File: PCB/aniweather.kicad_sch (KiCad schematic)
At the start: 4 parts, among them SW1 SW_SPDT

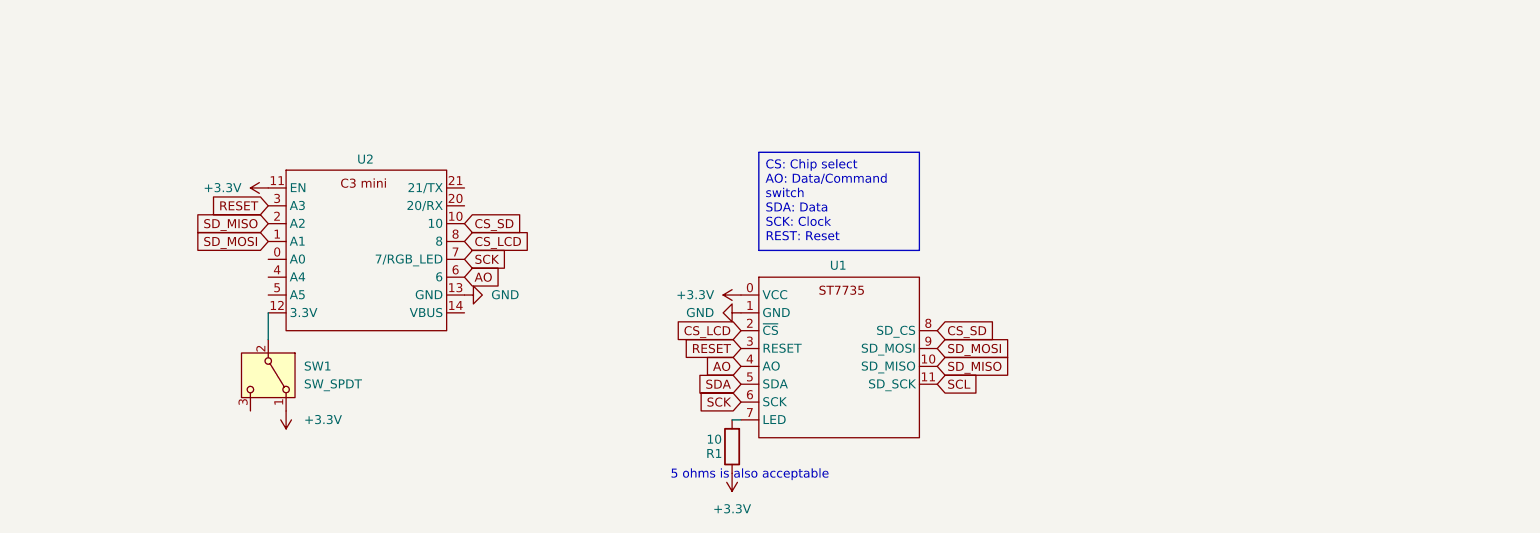
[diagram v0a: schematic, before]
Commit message: Further improvements
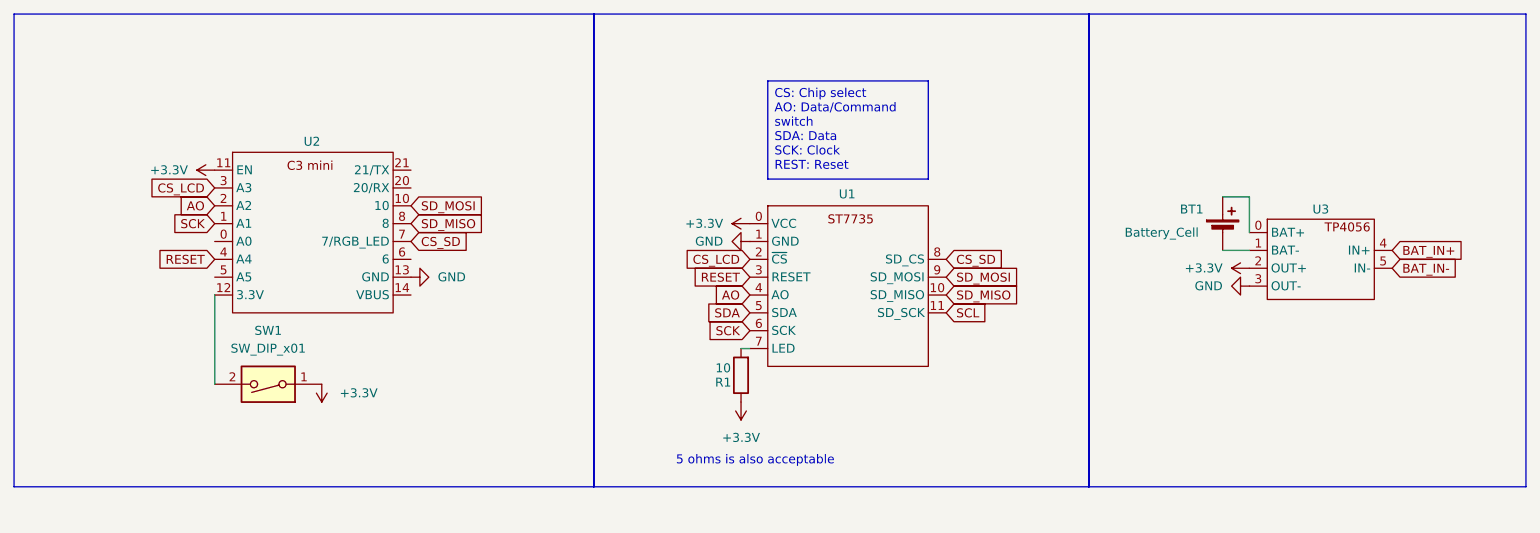
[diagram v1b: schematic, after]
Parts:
- removed SW1: SW_SPDT, symbol Switch:SW_SPDT
- added BT1: Battery_Cell, TestPoint:TestPoint_2Pads_Pitch5.08mm_Drill1.3mm, symbol Device:Battery_Cell
- added SW1: SW_DIP_x01, Button_Switch_THT:SW_DIP_SPSTx01_Slide_9.78x4.72mm_W7.62mm_P2.54mm, symbol Switch:SW_DIP_x01
- added U3: ~, asylum:TP4056, symbol asylum:TP4056
- R1: footprint (none) -> Resistor_THT:R_Axial_DIN0207_L6.3mm_D2.5mm_P10.16mm_Horizontal
- U1: footprint (none) -> asylum:ST7735
- U2: footprint (none) -> asylum:C3 mini
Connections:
- net +3.3V: now also SW1.1, U3.2 (OUT+)
- net AO: now also U2.2 (A2); no longer U2.6
- net CS_LCD: now also U2.3 (A3); no longer U2.8
- net CS_SD: now also U2.7 (7/RGB_LED); no longer U2.10
- net GND: now also U3.3 (OUT-)
- net RESET: now also U2.4 (A4); no longer U2.3 (A3)
- net SCK: now also U2.1 (A1); no longer U2.7 (7/RGB_LED)
- net SD_MISO: now also U2.8; no longer U2.2 (A2)
- net SD_MOSI: now also U2.10; no longer U2.1 (A1)
- net at U2.12 (3.3V): now also SW1.2
- new net: BT1.1 (+), U3.0 (BAT+)
- new net: BT1.2 (-), U3.1 (BAT-)
- new net BAT_IN+: U3.4 (IN+)
- new net BAT_IN-: U3.5 (IN-)
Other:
- moved on the sheet: R1, U1, U2

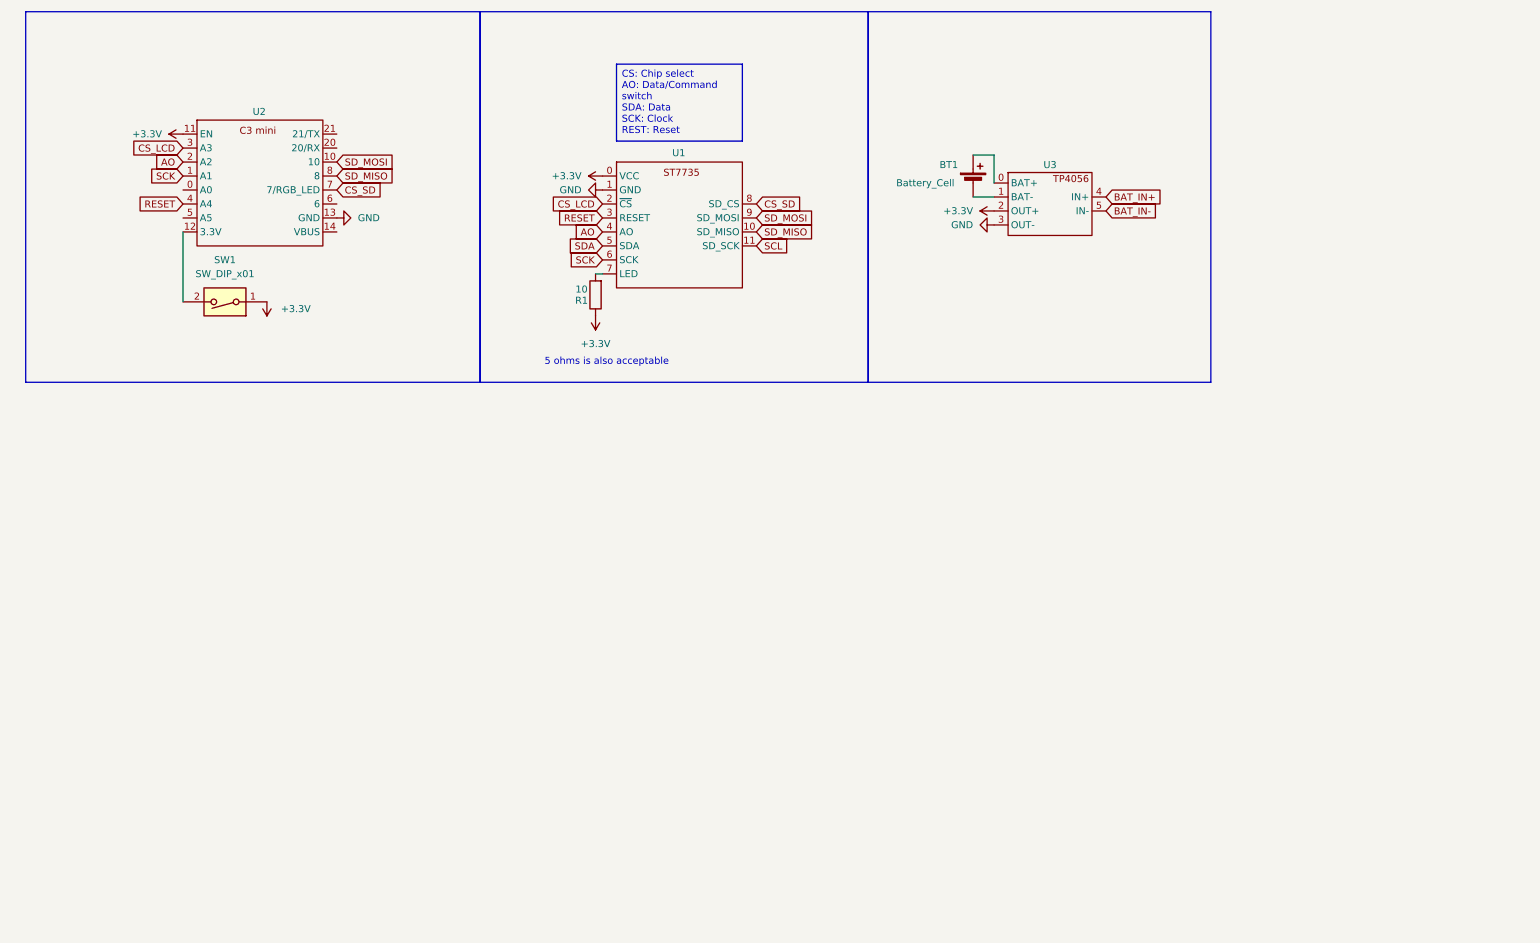
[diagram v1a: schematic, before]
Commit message: Saber plus PCB start
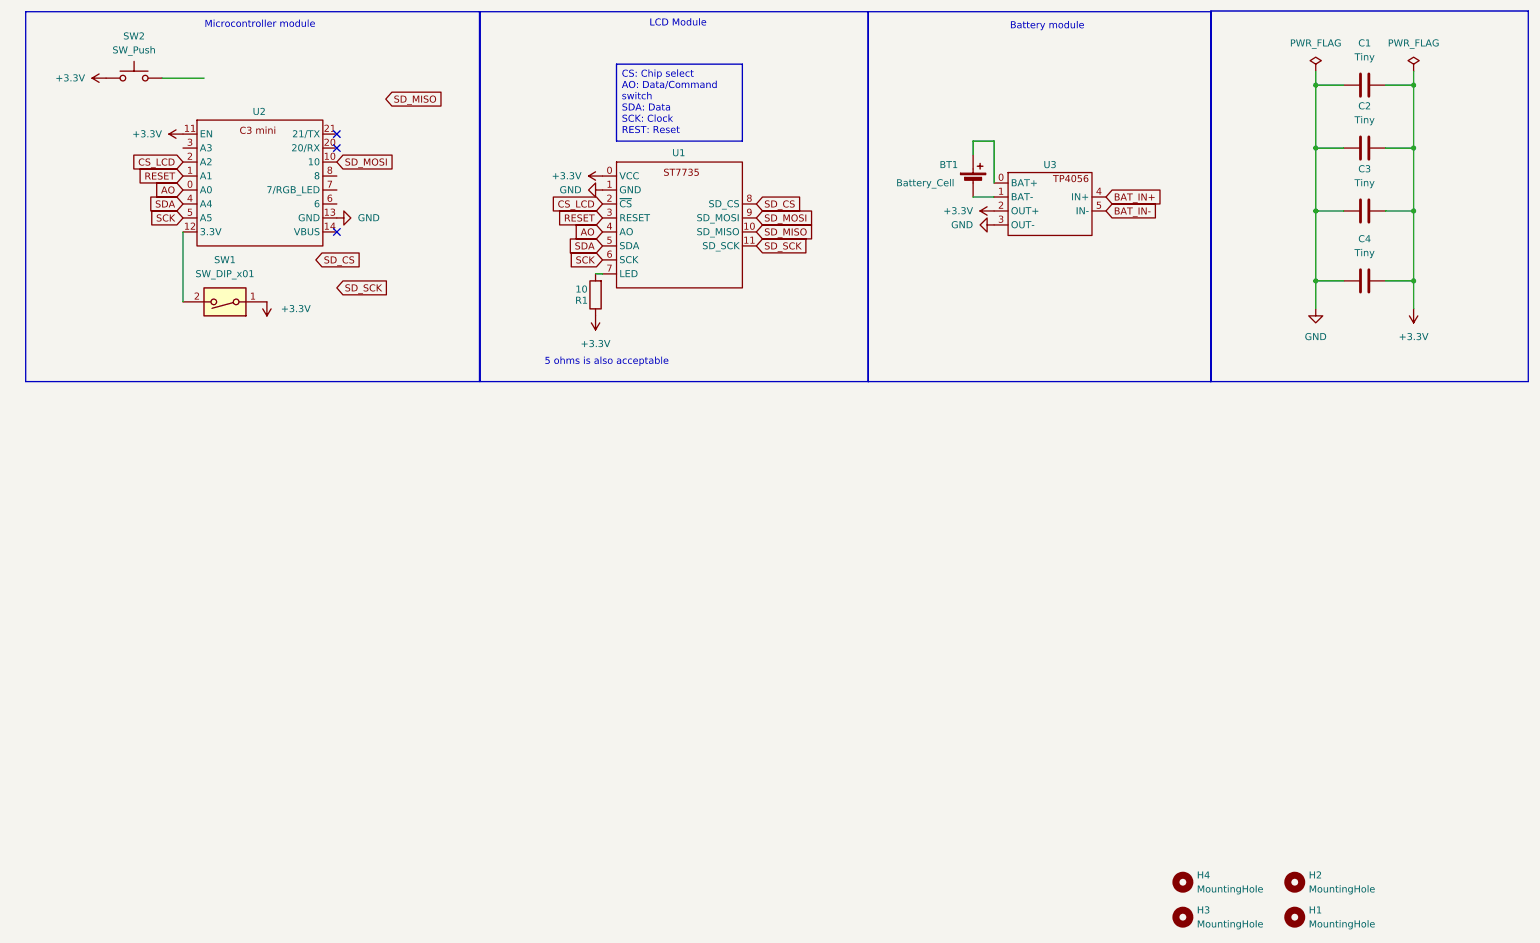
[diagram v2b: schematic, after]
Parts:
- added C1, C2, C3, C4: Tiny, Capacitor_THT:C_Disc_D5.0mm_W2.5mm_P2.50mm, symbol Device:C
- added H1, H2, H3, H4: MountingHole, MountingHole:MountingHole_3.2mm_M3, symbol Mechanical:MountingHole
- added SW2: SW_Push, Button_Switch_THT:SW_PUSH_6mm, symbol Switch:SW_Push
- U2: footprint asylum:C3 mini -> asylum:WEMOS_C1_mini
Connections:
- net +3.3V: now also C1.2, C2.2, C3.2, C4.2, SW2.1
- net AO: now also U2.0 (A0); no longer U2.2 (A2)
- net CS_LCD: now also U2.2 (A2); no longer U2.3 (A3)
- net GND: now also C1.1, C2.1, C3.1, C4.1
- net RESET: now also U2.1 (A1); no longer U2.4 (A4)
- net SCK: now also U2.5 (A5); no longer U2.1 (A1)
- net SDA: now also U2.4 (A4)
- net SD_MISO: no longer U2.8
- net CS_SD: no longer names the net of U2.7 (7/RGB_LED)
- net CS_SD: no longer U1.8 (SD_CS)
- net SCL renamed SD_SCK
- new net SD_CS: U1.8 (SD_CS)
- no-connect marks 0 -> 3
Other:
- note added: "Battery module"
- note added: "LCD Module"
- note added: "Microcontroller module"

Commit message: V1.0
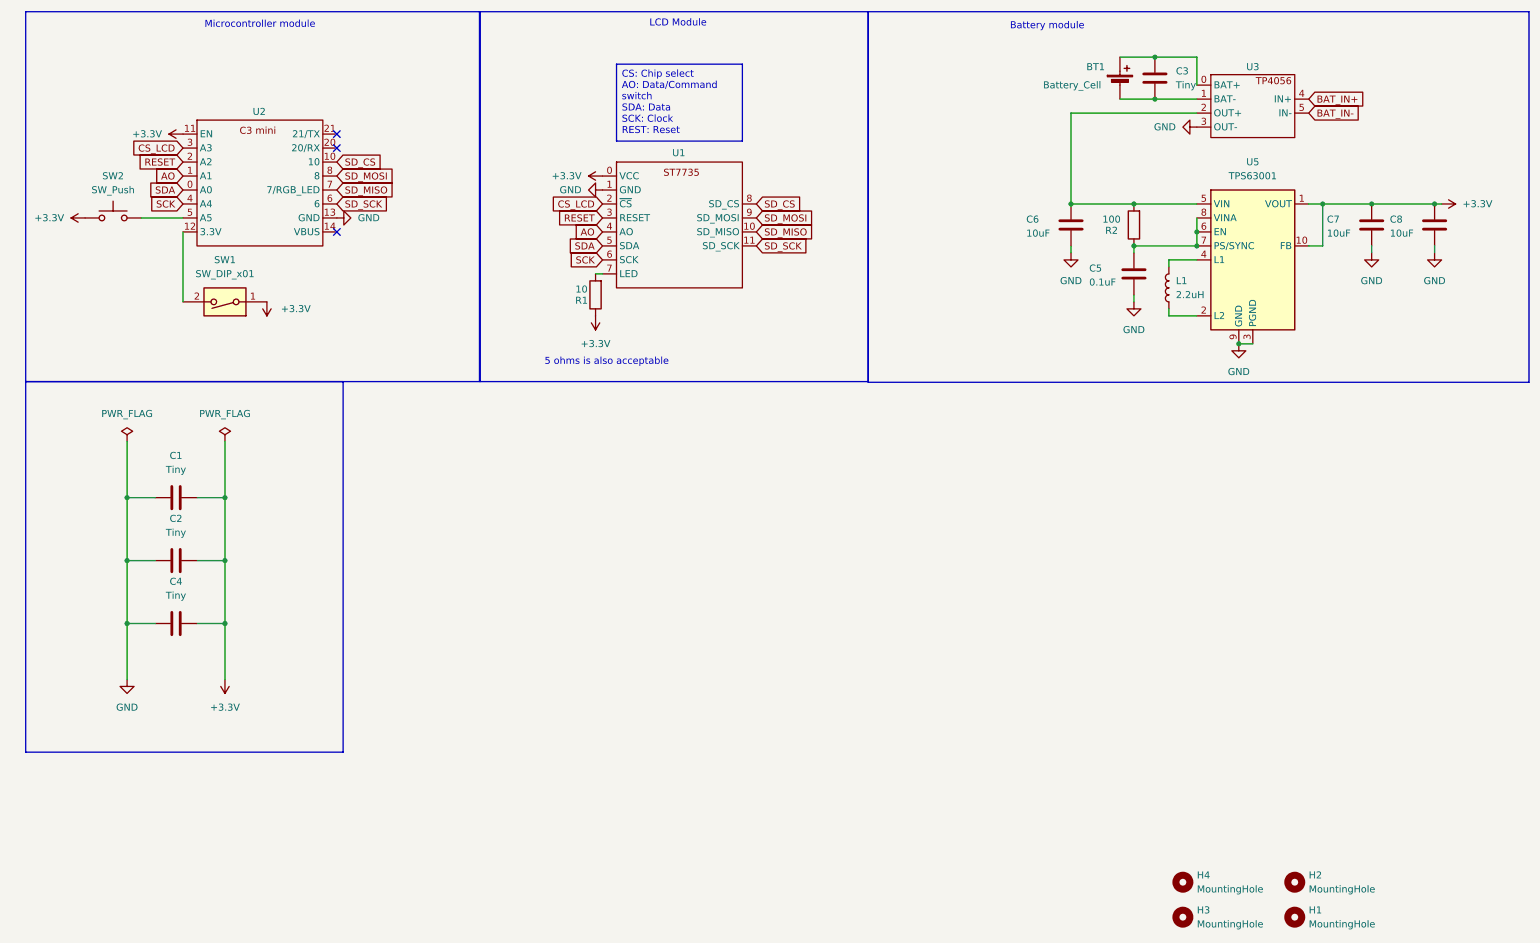
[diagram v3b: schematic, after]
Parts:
- added C5: 0.1uF, Capacitor_THT:C_Disc_D5.0mm_W2.5mm_P2.50mm, symbol Device:C
- added C6, C7, C8: 10uF, Capacitor_THT:C_Disc_D5.0mm_W2.5mm_P2.50mm, symbol Device:C
- added L1: 2.2uH, Inductor_SMD:L_1210_3225Metric, symbol Device:L
- added R2: 100, Resistor_THT:R_Axial_DIN0207_L6.3mm_D2.5mm_P10.16mm_Horizontal, symbol Device:R
- added U5: TPS63001, Package_SON:Texas_DRC0010J_ThermalVias, symbol Regulator_Switching:TPS63001
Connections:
- net +3.3V: now also C4.1, C7.1, C8.1, U5.1 (VOUT), U5.10 (FB); no longer C3.2, C4.2, U3.2 (OUT+)
- net AO: now also U2.1 (A1); no longer U2.0 (A0)
- net CS_LCD: now also U2.3 (A3); no longer U2.2 (A2)
- net GND: now also C4.2, C5.2, C6.2, C7.2, C8.2, U5.11 (PGND), U5.3 (PGND), U5.9 (GND); no longer C3.1, C4.1
- net RESET: now also U2.2 (A2); no longer U2.1 (A1)
- net SCK: now also U2.4 (A4); no longer U2.5 (A5)
- net SDA: now also U2.0 (A0); no longer U2.4 (A4)
- net SD_CS: now also U2.10
- net SD_MISO: now also U2.7 (7/RGB_LED)
- net SD_MOSI: now also U2.8; no longer U2.10
- net SD_SCK: now also U2.6
- net at SW2.2: now also U2.5 (A5)
- net at BT1.1 (+), U3.0 (BAT+): now also C3.1
- net at BT1.2 (-), U3.1 (BAT-): now also C3.2
- new net: C5.1, R2.1, U5.6 (EN), U5.7 (PS/SYNC), U5.8 (VINA)
- new net: L1.1, U5.2 (L2)
- new net: L1.2, U5.4 (L1)
- new net: C6.1, R2.2, U3.2 (OUT+), U5.5 (VIN)
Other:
- moved on the sheet: BT1, C1, C2, C3, C4, SW2, U3

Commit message: Fix some small issues
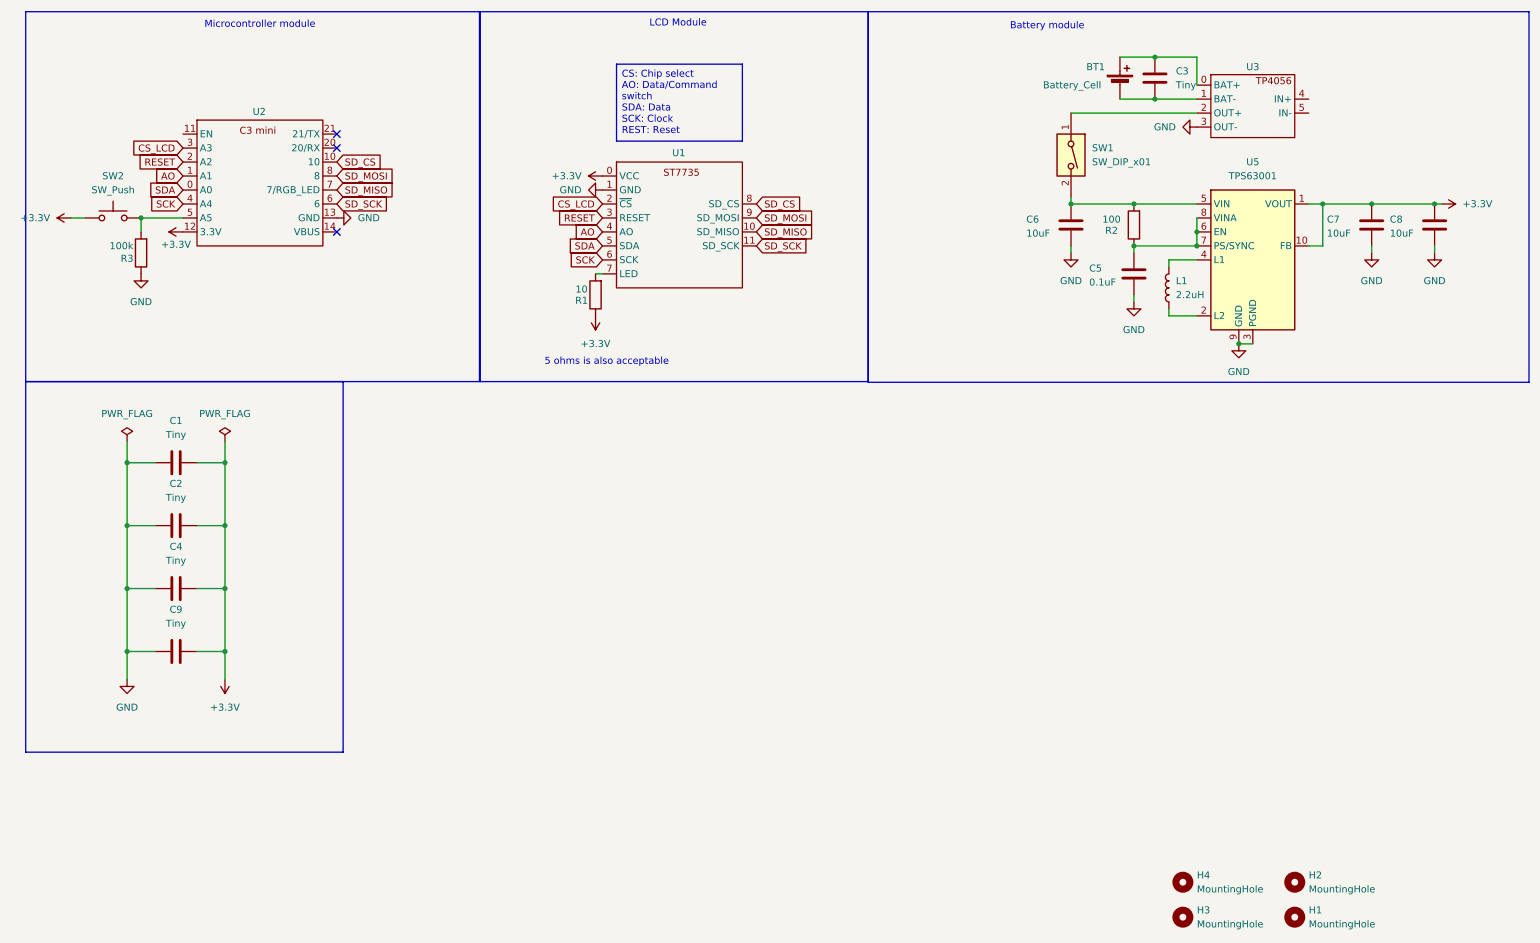
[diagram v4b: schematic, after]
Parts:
- added C9: Tiny, Capacitor_THT:C_Disc_D5.0mm_W2.5mm_P2.50mm, symbol Device:C
- added R3: 100k, Resistor_THT:R_Axial_DIN0207_L6.3mm_D2.5mm_P10.16mm_Horizontal, symbol Device:R
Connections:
- net +3.3V: now also U2.12 (3.3V), C9.1; no longer SW1.1, U2.11 (EN)
- net GND: now also C9.2, R3.1
- net at C6.1, R2.2, U5.5 (VIN): now also SW1.2; no longer U3.2 (OUT+)
- net at SW2.2, U2.5 (A5): now also R3.2
- net BAT_IN+: no longer names the net of U3.4 (IN+)
- net BAT_IN-: no longer names the net of U3.5 (IN-)
- new net: SW1.1, U3.2 (OUT+)
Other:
- moved on the sheet: C1, C2, C4, SW1
